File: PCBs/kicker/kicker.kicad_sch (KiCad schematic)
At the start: 12 parts, among them Q1 CSD19534Q5A, U1 UCC27624DR

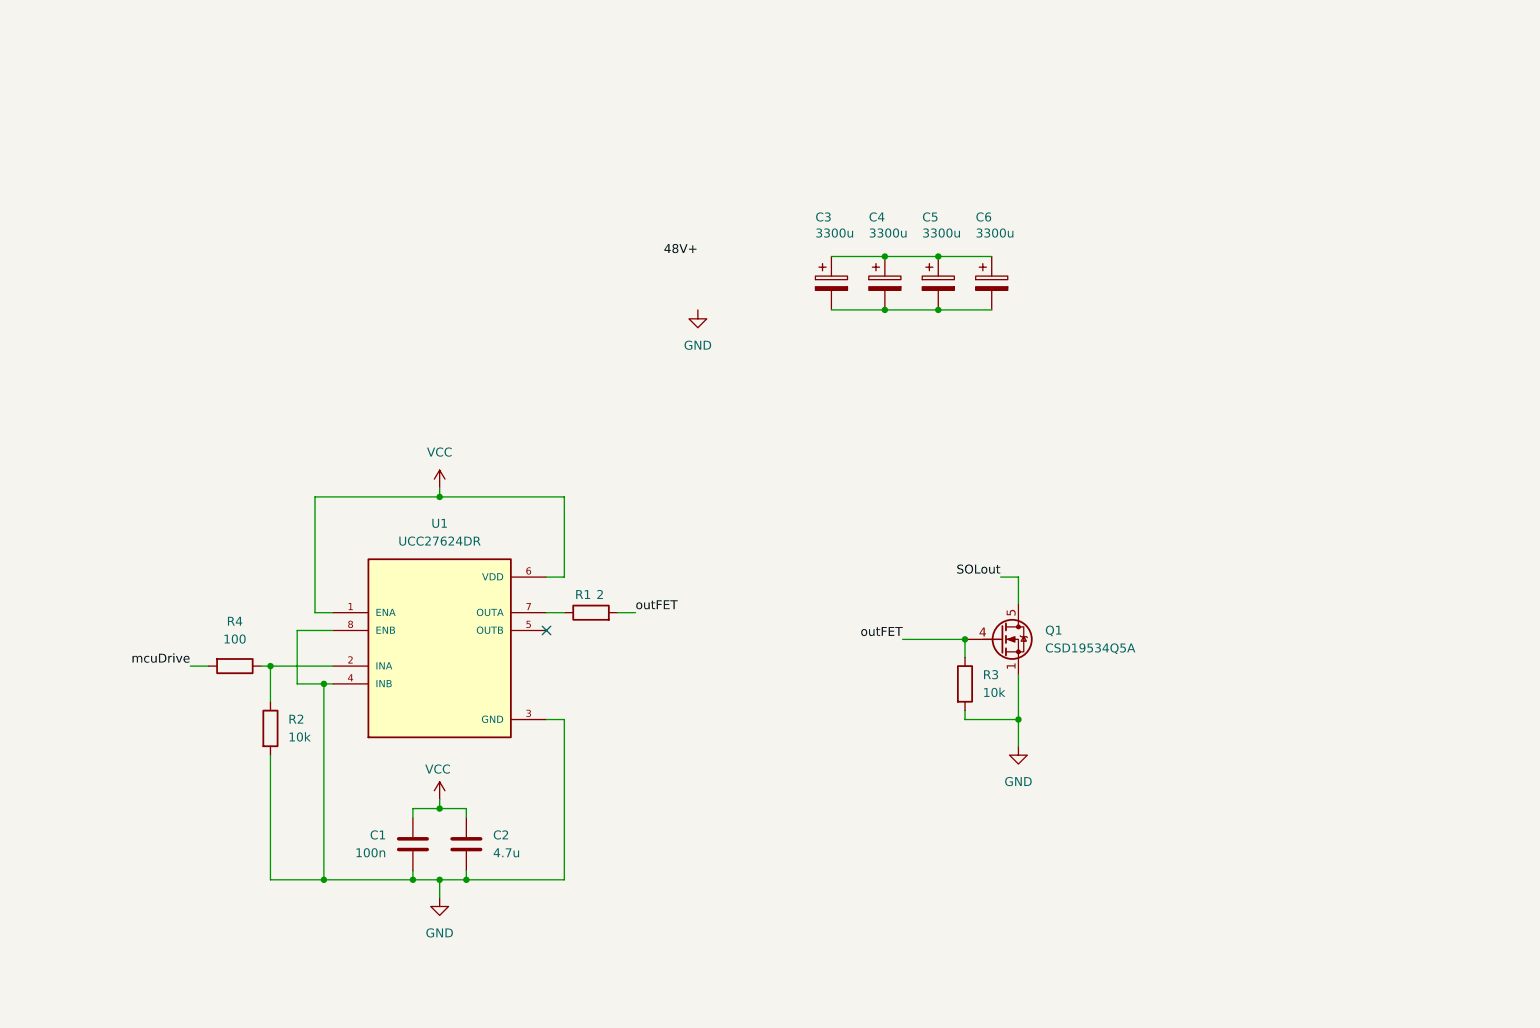
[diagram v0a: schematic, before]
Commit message: kicker v0.1
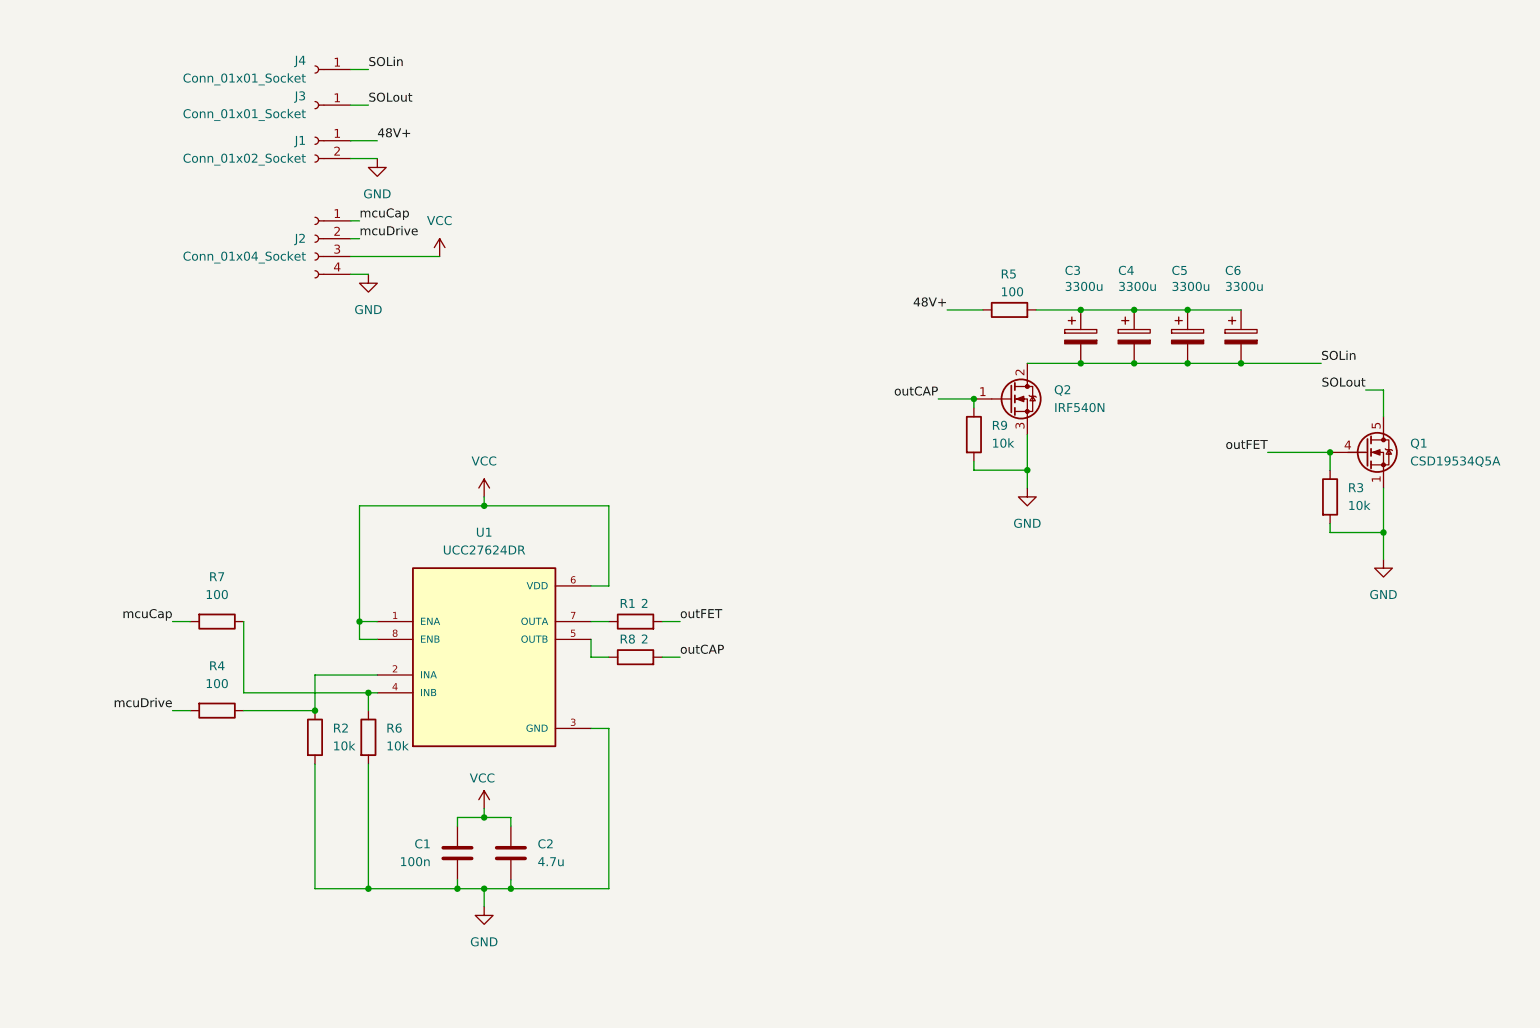
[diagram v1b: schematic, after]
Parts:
- added J1: Conn_01x02_Socket, Connector_JST:JST_XH_S2B-XH-A-1_1x02_P2.50mm_Horizontal, symbol Connector:Conn_01x02_Socket
- added J2: Conn_01x04_Socket, Connector_JST:JST_XH_S4B-XH-A-1_1x04_P2.50mm_Horizontal, symbol Connector:Conn_01x04_Socket
- added J3, J4: Conn_01x01_Socket, Connector_Wire:SolderWirePad_1x01_SMD_5x10mm, symbol Connector:Conn_01x01_Socket
- added Q2: IRF540N, Package_TO_SOT_THT:TO-220-3_Horizontal_TabDown, symbol Transistor_FET:IRF540N
- added R5: 100, Package_TO_SOT_SMD:TO-263-2, symbol Device:R
- added R6, R9: 10k, Resistor_SMD:R_0603_1608Metric, symbol Device:R
- added R7: 100, Resistor_SMD:R_0603_1608Metric, symbol Device:R
- added R8: 2, Resistor_SMD:R_0805_2012Metric, symbol Device:R
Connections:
- net 48V+: now also J1.1 (Pin_1), R5.1
- net GND: now also J1.2 (Pin_2), J2.4 (Pin_4), Q2.3 (S), R6.2, R9.2; no longer U1.4 (INB), U1.8 (ENB)
- net SOLout: now also J3.1 (Pin_1)
- net VCC: now also U1.8 (ENB), J2.3 (Pin_3)
- net mcuDrive: now also J2.2 (Pin_2)
- net at C3.1, C4.1, C5.1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: now also R5.2
- net SOLin: now reaches C3.2, C4.2, C5.2, C6.2
- net SOLin: now also J4.1 (Pin_1), Q2.2 (D)
- net at U1.5 (OUTB): now also R8.1
- new net: R6.1, R7.1, U1.4 (INB)
- new net mcuCap: J2.1 (Pin_1), R7.2
- new net outCAP: Q2.1 (G), R8.2, R9.1
- no-connect marks 1 -> 0
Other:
- moved on the sheet: C1, C2, C3, C4, C5, C6, Q1, R1, R2, R3, R4, U1

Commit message: ee
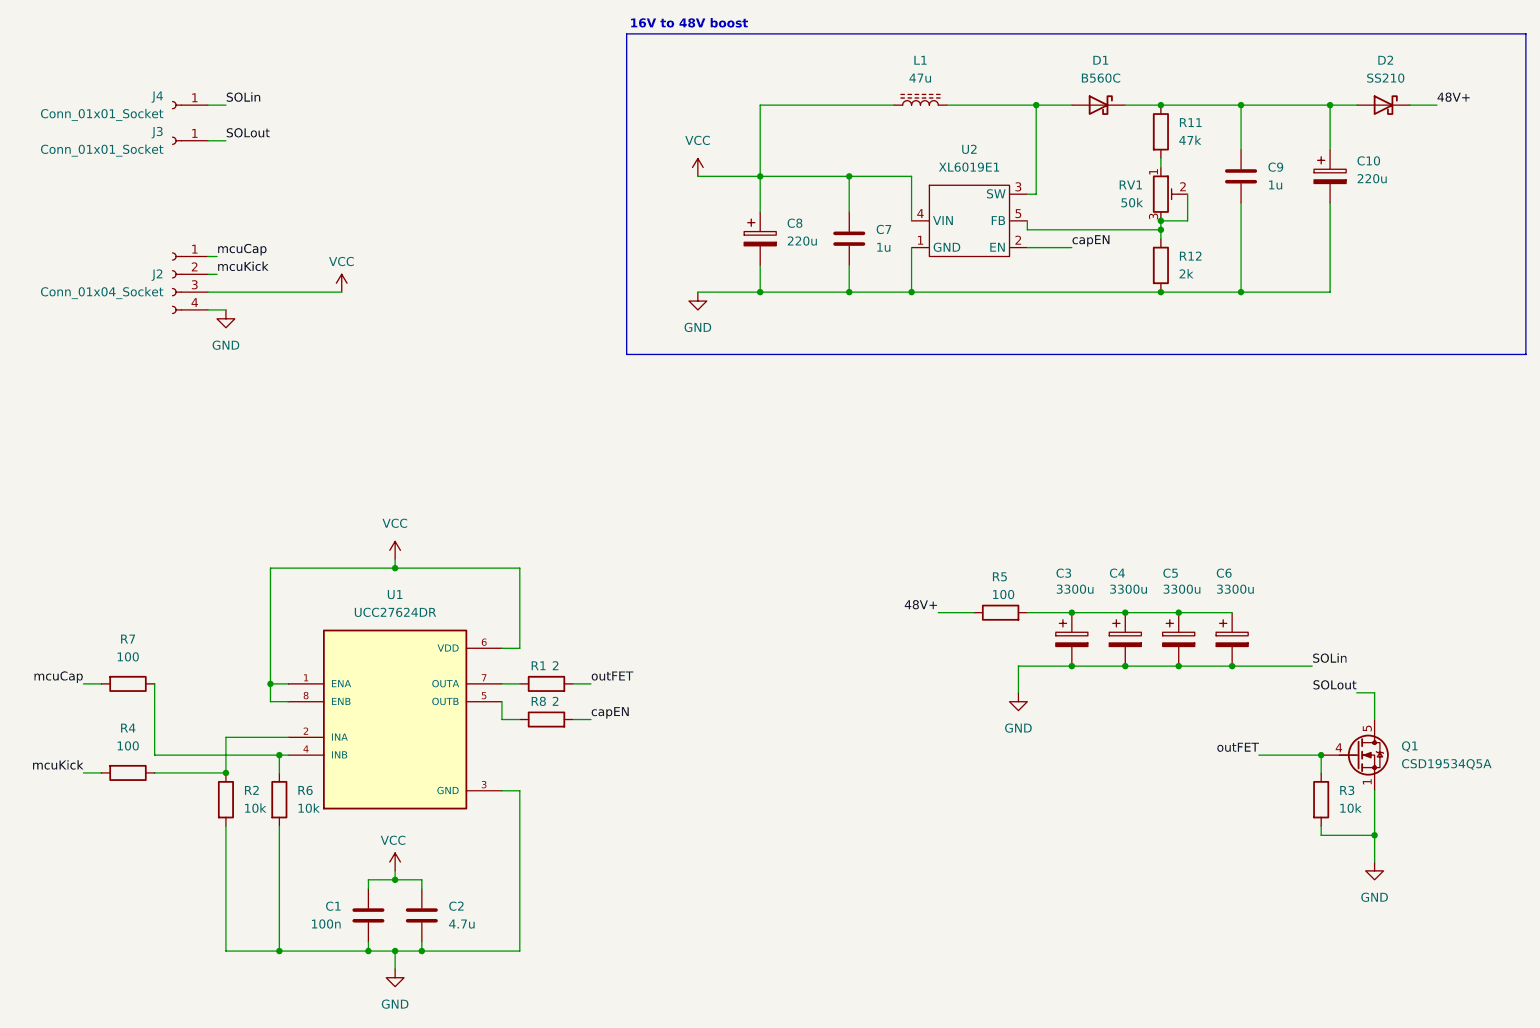
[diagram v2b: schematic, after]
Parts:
- removed J1: Conn_01x02_Socket, Connector_JST:JST_XH_S2B-XH-A-1_1x02_P2.50mm_Horizontal, symbol Connector:Conn_01x02_Socket
- removed Q2: IRF540N, Package_TO_SOT_THT:TO-220-3_Horizontal_TabDown, symbol Transistor_FET:IRF540N
- removed R9: 10k, Resistor_SMD:R_0603_1608Metric, symbol Device:R
- added C10, C8: 220u, Capacitor_SMD:CP_Elec_10x10.5, symbol Device:C_Polarized
- added C7, C9: 1u, Capacitor_SMD:C_1206_3216Metric, symbol Device:C
- added D1: B560C, digikey-footprints:DO-214AB, symbol Device:D_Schottky
- added D2: SS210, Diode_SMD:D_SMA, symbol Device:D_Schottky
- added L1: 47u, Inductor_SMD:L_Sunlord_MWSA1206S-470, symbol Device:L_Ferrite
- added R11: 47k, Resistor_SMD:R_0603_1608Metric, symbol Device:R
- added R12: 2k, Resistor_SMD:R_0603_1608Metric, symbol Device:R
- added RV1: 50k, Potentiometer_THT:Potentiometer_Bourns_3296W_Vertical, symbol Device:R_Potentiometer_Trim
- added U2: XL6019E1, Package_TO_SOT_SMD:TO-263-5_TabPin3, symbol New_Library:XL6019E1
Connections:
- net SOLin is gone; now on net GND: C3.2, C4.2, C5.2, C6.2, J4.1 (Pin_1)
- net 48V+: now also D2.1 (K)
- net GND: now also C10.2, C7.2, C8.2, C9.2, R12.2, U2.1 (GND)
- net VCC: now also C7.1, C8.1, L1.1, U2.4 (VIN)
- net mcuDrive renamed mcuKick
- net outCAP renamed capEN
- net capEN: now also U2.2 (EN)
- new net: C10.1, C9.1, D1.1 (K), D2.2 (A), R11.1
- new net: D1.2 (A), L1.2, U2.3 (SW)
- new net: R12.1, RV1.2, RV1.3, U2.5 (FB)
- new net: R11.2, RV1.1
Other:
- note added: "16V to 48V boost"
- moved on the sheet: C1, C2, C3, C4, C5, C6, J2, J3, J4, Q1, R1, R2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
